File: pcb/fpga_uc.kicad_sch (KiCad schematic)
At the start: 1 part

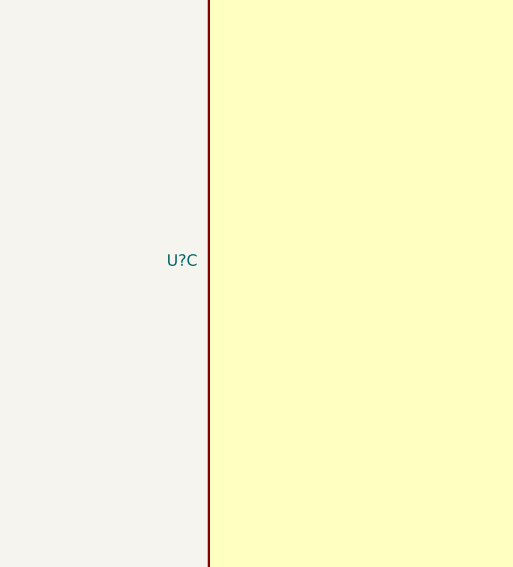
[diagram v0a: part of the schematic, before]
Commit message: kicad said I needed to save
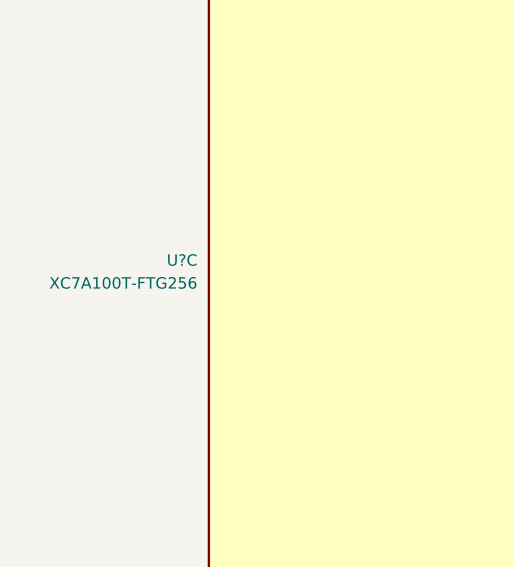
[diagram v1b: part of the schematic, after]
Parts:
- U?: value (none) -> XC7A100T-FTG256
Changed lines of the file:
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@@
       (effects (font (size 1.27 1.27)) (justify right))
     )
-    (property "Value" "" (id 1) (at 67.31 81.9149 0)
+    (property "Value" "XC7A100T-FTG256" (id 1) (at 67.31 81.9149 0)
       (effects (font (size 1.27 1.27)) (justify right))
     )
